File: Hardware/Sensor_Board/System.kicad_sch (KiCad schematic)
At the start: 35 parts, among them J301 RJ45, J302 TC2030, J303 PicoBlade, SW301 Reset, U301 ICE40UL1K-CM36AI, U302 TPD4E02B04, U303 TPD4E02B04, U304 TPD4E02B04, U305 N25Q032A, Y301 ASCO

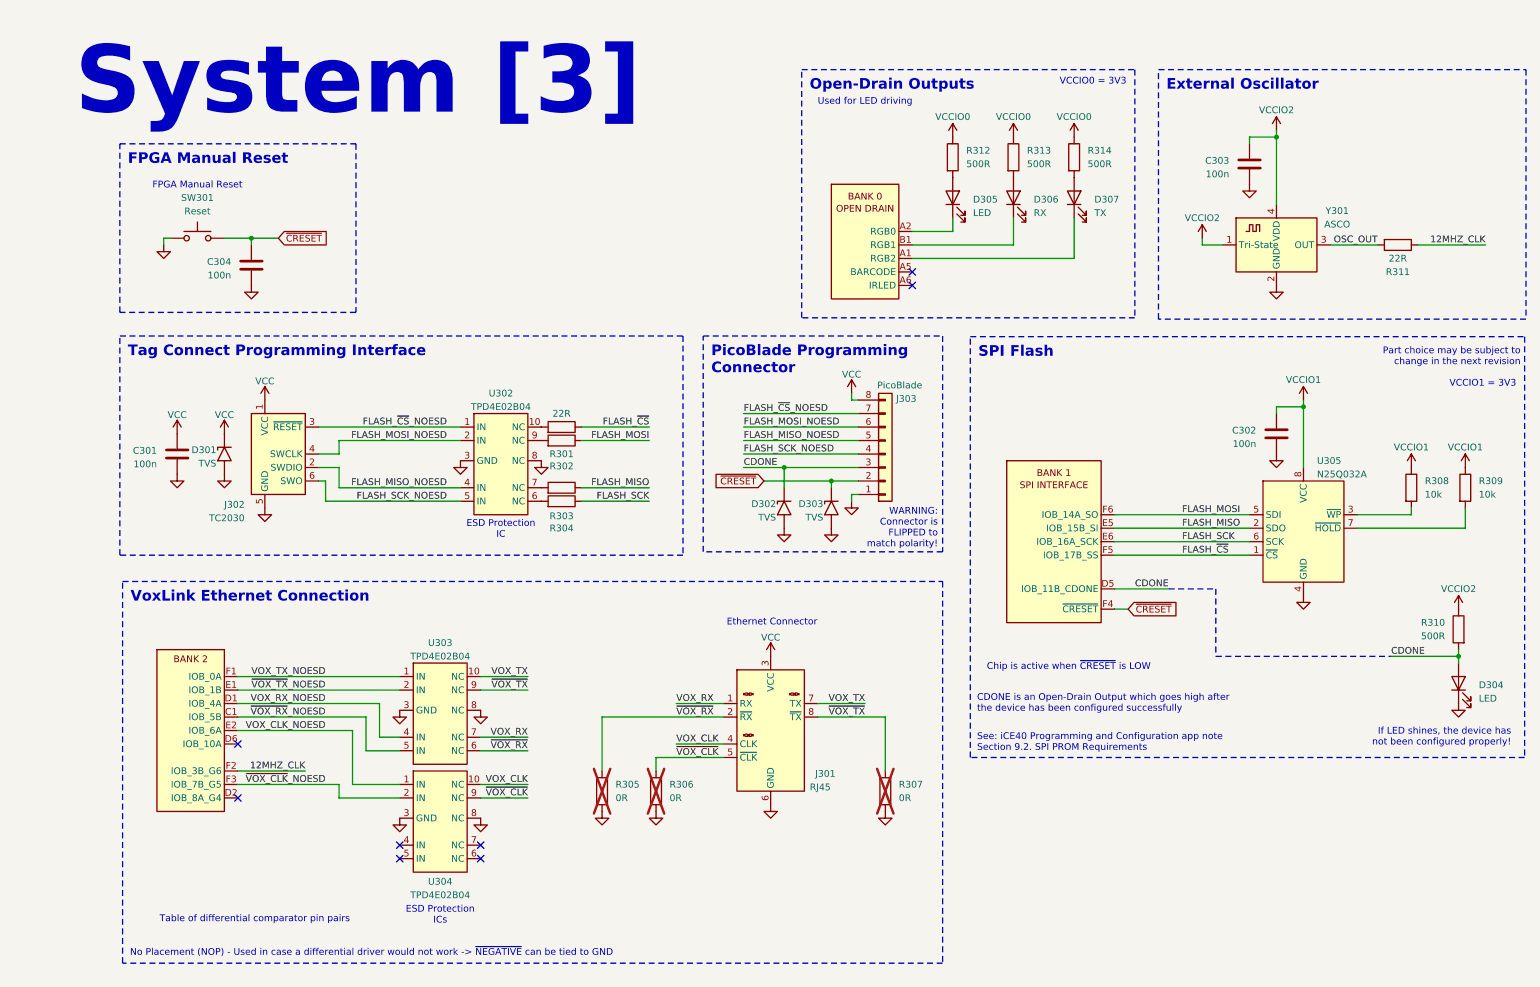
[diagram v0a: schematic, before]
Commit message: Added documantation regarding the programmer board and updated the PDF schematics.
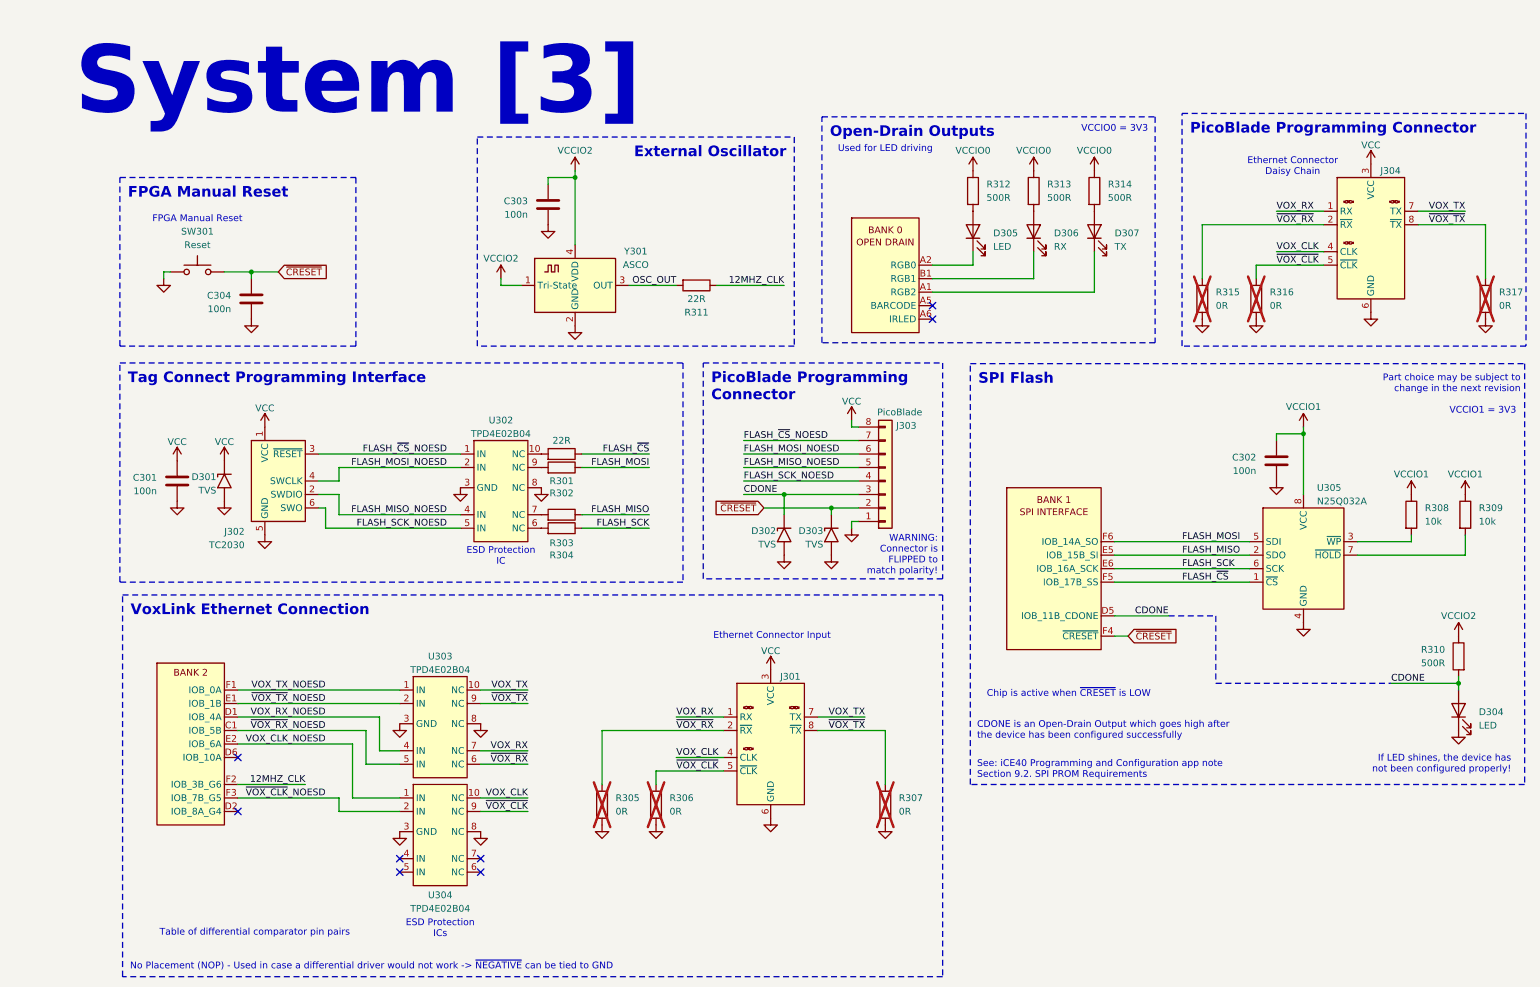
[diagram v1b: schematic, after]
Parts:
- removed J301: RJ45, rj45_molex_unshielded:CONN_855035-101_MOL, symbol rj45_molex_unshielded:RJ45_Molex_Unshielded
- added J301: RJ45_Input, rj45_molex_unshielded:CONN_855035-101_MOL, symbol rj45_molex_unshielded:RJ45_Molex_Unshielded_Input
- added J304: RJ45_Output, rj45_molex_unshielded:CONN_855035-101_MOL, symbol rj45_molex_unshielded:RJ45_Molex_Unshielded_Output
- added R315, R316, R317: 0R, symbol Device:R
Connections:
- net GND: now also J301.6 (GND), J304.6 (GND), R315.2, R316.2, R317.2
- net VCC: now also J301.3 (VCC), J304.3 (VCC)
- net VOX_CLK: now also J301.4 (CLK), J304.4 (CLK)
- net VOX_RX: now also J301.1 (RX), J304.1 (RX)
- net VOX_TX: now also J301.7 (TX), J304.7 (TX)
- net ~{VOX_CLK}: now also J301.5 (~{CLK}), J304.5 (~{CLK}), R316.1
- net ~{VOX_RX}: now also J301.2 (~{RX}), J304.2 (~{RX}), R315.1
- net ~{VOX_TX}: now also J301.8 (~{TX}), J304.8 (~{TX}), R317.1
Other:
- note added: "Ethernet Connector Daisy Chain"
- note added: "Ethernet Connector Input"
- note removed: "Ethernet Connector"
- moved on the sheet: C301, C302, C303, C304, D301, D302, D303, D304, D305, D306, D307, J302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

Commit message: Pushing before updating KiCad
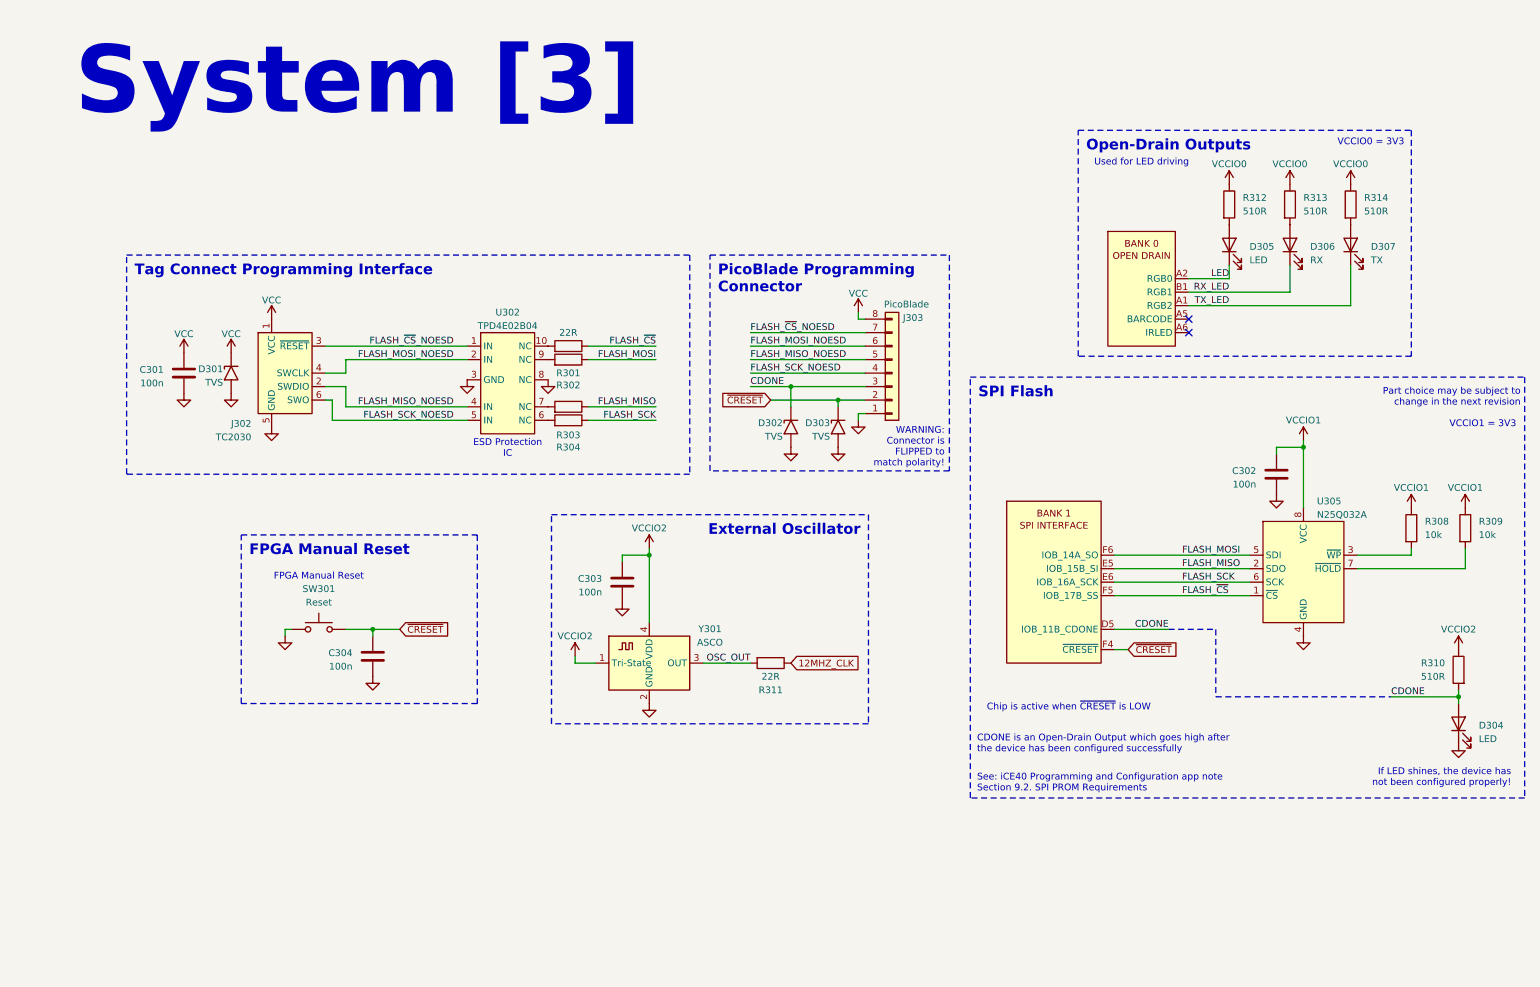
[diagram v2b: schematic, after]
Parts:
- removed J301: RJ45_Input, rj45_molex_unshielded:CONN_855035-101_MOL, symbol rj45_molex_unshielded:RJ45_Molex_Unshielded_Input
- removed J304: RJ45_Output, rj45_molex_unshielded:CONN_855035-101_MOL, symbol rj45_molex_unshielded:RJ45_Molex_Unshielded_Output
- removed R305, R306, R307, R315, R316, R317: 0R, symbol Device:R
- removed unit 2 of U301
- removed U303, U304: TPD4E02B04, Package_SON:USON-10_2.5x1.0mm_P0.5mm, symbol Custom_VoxLink_Symbols:TPD4E02B04DQA
- D304, D305, D306, D307: footprint (none) -> LED_SMD:LED_0603_1608Metric
- R308, R309: footprint (none) -> Resistor_SMD:R_0402_1005Metric
- R310, R312, R313, R314: value 500R -> 510R; footprint (none) -> Resistor_SMD:R_0402_1005Metric
- SW301: footprint (none) -> Button_Switch_SMD:SW_Push_SPST_NO_Alps_SKRK
- U301: footprint Package_BGA:UCBGA-36_2.5x2.5mm_Layout6x6_P0.4mm -> Custom_VoxLink_Footprints:ICE40UL1K_UCBGA-36
- U305: footprint (none) -> Custom_VoxLink_Footprints:U-PDFN-8
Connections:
- net LED: now reaches D305.1 (K), U301.A2 (RGB0)
- net TX_LED: now reaches D307.1 (K), U301.A1 (RGB2)
- net RX_LED: now reaches D306.1 (K), U301.B1 (RGB1)
- no-connect marks 8 -> 2
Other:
- note removed: "ESD Protection ICs"
- note removed: "Ethernet Connector Daisy Chain"
- note removed: "Ethernet Connector Input"
- note removed: "No Placement (NOP) - Used in case a differential driver would not work -> ~{NEGATIVE} can be tied to GND"
- note removed: "Table of differential comparator pin pairs"
- moved on the sheet: C301, C302, C303, C304, D301, D302, D303, D304, D305, D306, D307, J302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
